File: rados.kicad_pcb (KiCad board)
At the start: 2 copper layers, 83.2 x 106 mm, 156 parts, among them J1 HEADER, J10 STEPSTICK, J11 STEPSTICK, J12 STEPSTICK, J13 MICROSD_SLOT_TFP09-2-12B, J2 HEADER, J3 HEADER, J4 STEPSTICK, J5 STEPSTICK, J6 STEPSTICK, J7 HEADER, J8 HEADER, J9 HEADER, P1 CONN_01X02, P10 CONN_01X04, P11 CONN_01X04, P12 CONN_01X04, P13 EXT_SD, P14 LCD, P15 LIMIT_SWITCHES, P16 LIMIT_SWITCHES_V, P17 CONN_01X03, P18 CONN_01X03, P19 CONN_01X03, P2 CONN_01X02, P20 CONN_01X03, P21 THERMISTORS, P22 CONN_01X05, P3 CONN_01X02, P4 CONN_01X02, P5 HP_MOSFETS, P6 MP_MOSFETS, P7 CONN_02X04, P8 CONN_01X04, P9 CONN_01X04, Q1 2N7002P, Q10 2N7002P, Q11 2N7002P, Q12 BC846BPDW1, Q13 BC846BPDW1, Q14 SI2318CDS-T1-GE3, Q15 IRFB7545PbF, Q16 2N7002P, Q17 2N7002P, Q18 BC846BPDW1, Q19 BC846BPDW1, Q2 2N7002P, Q20 SI2318CDS-T1-GE3, Q21 IRFB7545PbF, Q3 2N7002P, Q4 BC846BPDW1, Q5 BC846BPDW1, Q6 BC846BPDW1, Q7 IRFB7545PbF, Q8 SI2318CDS-T1-GE3, Q9 IRFB7545PbF, SW1 RESET, U1 MC34063, U2 24LC256, U3 ESP-12E

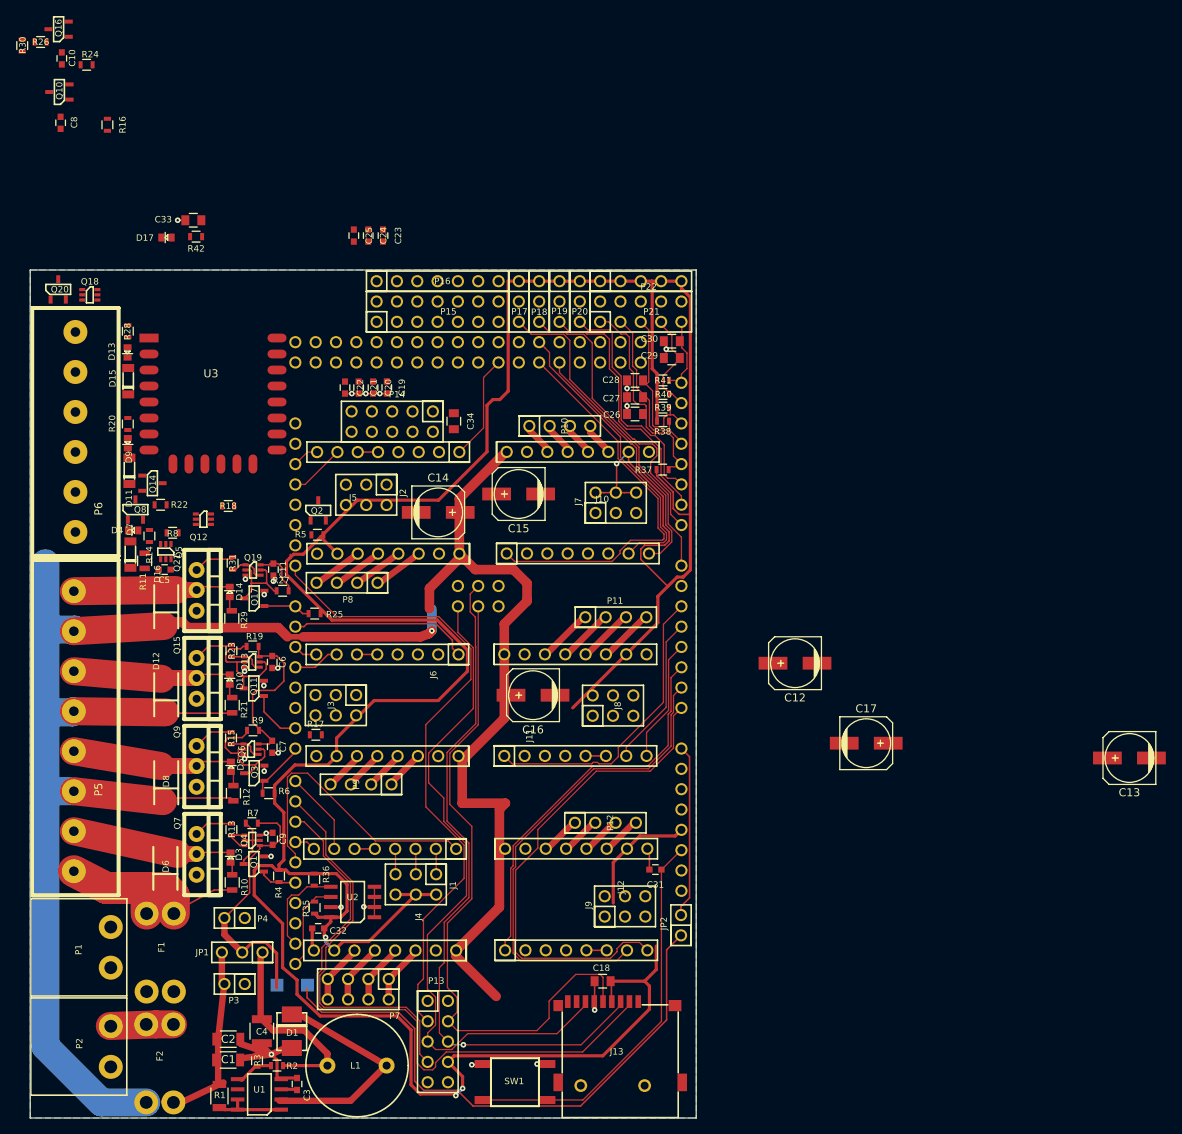
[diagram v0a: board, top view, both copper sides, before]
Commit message: Routing
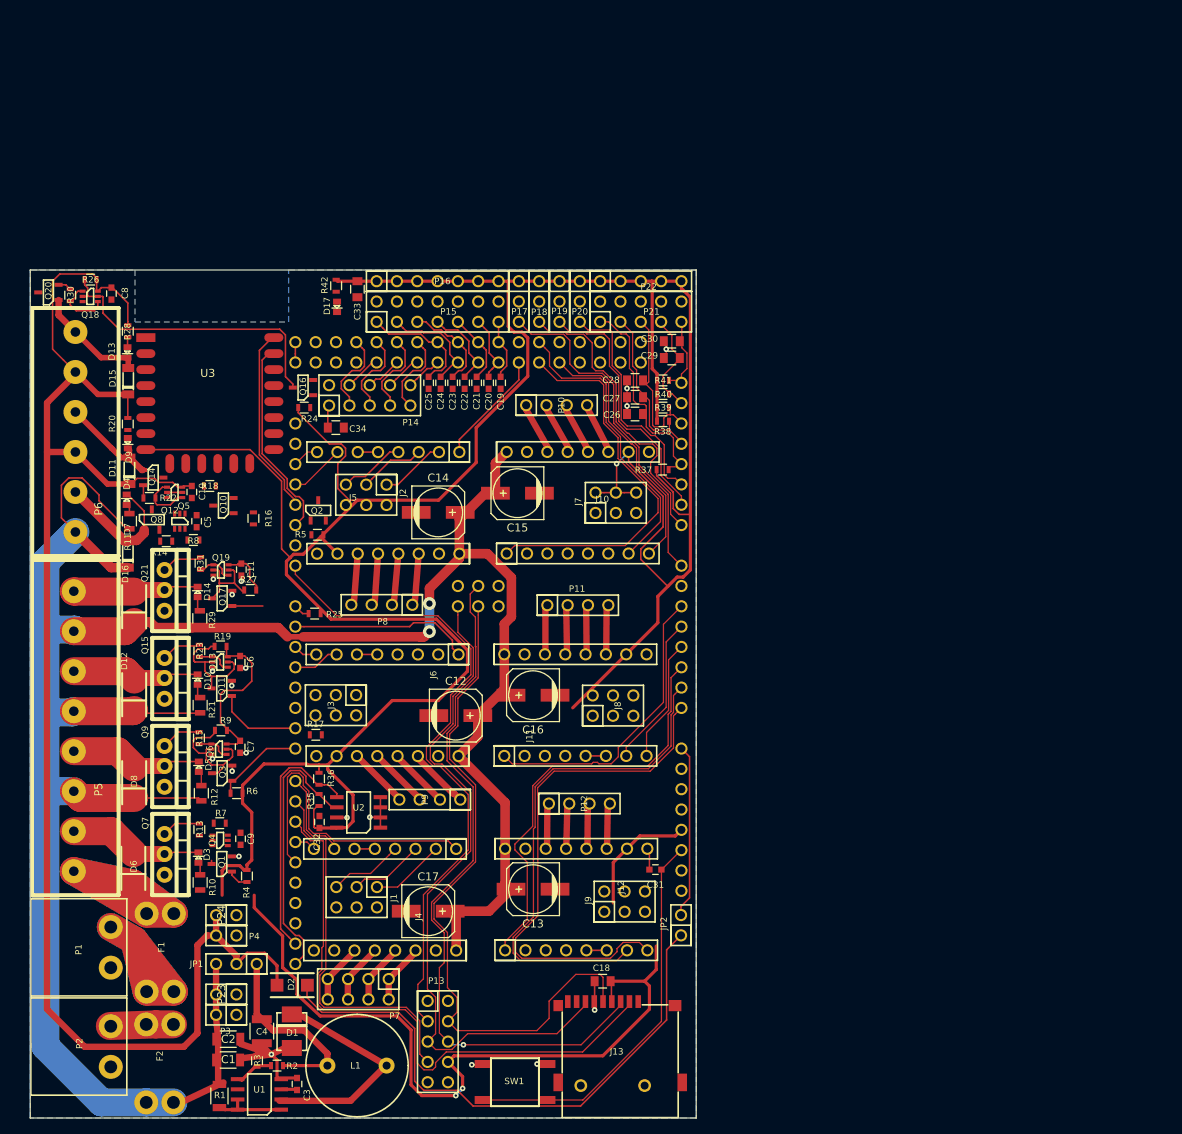
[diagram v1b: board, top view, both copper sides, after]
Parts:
- added P23: CONN_01X02, headers:CON_HDR_1x2_2.54mm, F.Cu at (95.5, 114.6)
- added P24: CONN_01X02, headers:CON_HDR_1x2_2.54mm, F.Cu at (95.5, 104.6)
- D2: moved to F.Cu
- moved C13 76.3 mm to (133.9, 101.4)
- moved C17 58.6 mm to (120.8, 104.2)
- moved C10 56.6 mm to (91.2, 51.8)
- moved Q10 55.6 mm to (95.2, 53.5)
- moved Q16 54.2 mm to (105.1, 38.7)
- moved R16 52.5 mm to (98.9, 55.0)
- moved R24 50.8 mm to (105.2, 41.2), turned to 180 degrees
- moved C12 42.9 mm to (124.2, 79.7), turned to 0 degrees
- moved R30 31.8 mm to (76.0, 27.1)
- moved R26 30.4 mm to (78.5, 25.2), turned to 0 degrees
- moved D17 23.0 mm to (109.3, 28.6), turned to 270 degrees
- moved C8 22.3 mm to (81.2, 26.9)
- moved C33 22.3 mm to (111.9, 26.4), turned to 270 degrees
- moved C25 20.6 mm to (120.8, 38.1)
- moved C24 20.5 mm to (122.3, 38.1)
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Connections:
- SHIELD1 pad 22: X- -> Net-(SHIELD1-Pad22)
- SHIELD1 pad 23: X+ -> Net-(SHIELD1-Pad23)
- SHIELD1 pad 24: Y- -> Net-(SHIELD1-Pad24)
- SHIELD1 pad 25: Y+ -> STATUS-LED
- SHIELD1 pad 26: Z- -> Net-(SHIELD1-Pad26)
- SHIELD1 pad 27: Z+ -> ENC-A
- SHIELD1 pad 28: Probe -> ENC-B
- SHIELD1 pad 29: STATUS-LED -> LCD-D5
- SHIELD1 pad 30: Net-(SHIELD1-Pad30) -> LCD-RS
- SHIELD1 pad 31: Net-(SHIELD1-Pad31) -> LCD-D6
- SHIELD1 pad 32: Net-(SHIELD1-Pad32) -> LCD-E
- SHIELD1 pad 33: LCD-D4 -> LCD-D7
- SHIELD1 pad 34: LCD-D7 -> LCD-D4
- SHIELD1 pad 35: LCD-D6 -> X-
- SHIELD1 pad 36: LCD-E -> X+
- SHIELD1 pad 37: LCD-D5 -> Y-
- SHIELD1 pad 38: LCD-RS -> Y+
- SHIELD1 pad 39: ENC-B -> Z-
- SHIELD1 pad 40: X-EN -> Z+
- SHIELD1 pad 41: ENC-A -> PROBE
- SHIELD1 pad 42: Net-(SHIELD1-Pad42) -> X-EN
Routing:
- net +12V: track 58.9 -> 218.9 mm
- net +3V3: track 430.2 -> 476.1 mm, vias 4 -> 3
- net Net-(F1-Pad1): track 0.00 -> 42.9 mm
- net Net-(Q16-Pad3): track 0.00 -> 37.7 mm
- net ESP-RX: track 0.00 -> 25.9 mm
- net Vheatbed: track 31.4 -> 55.8 mm
- net ESP-TX: track 0.00 -> 24.0 mm
- net SCL1: track 11.3 -> 34.5 mm
- net SDA1: track 12.0 -> 31.0 mm
- net Vsupply: track 298.5 -> 317.3 mm, vias 1 -> 2
- net MP-OUT1: track 0.00 -> 17.3 mm
- net X-: track 0.00 -> 14.8 mm
- net LP-OUT2: track 0.00 -> 14.0 mm
- net X+: track 0.00 -> 13.5 mm
- net LP-OUT1: track 0.00 -> 12.7 mm
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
